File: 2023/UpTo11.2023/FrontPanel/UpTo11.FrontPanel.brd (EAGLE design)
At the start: 88 x 78 mm, 16 parts

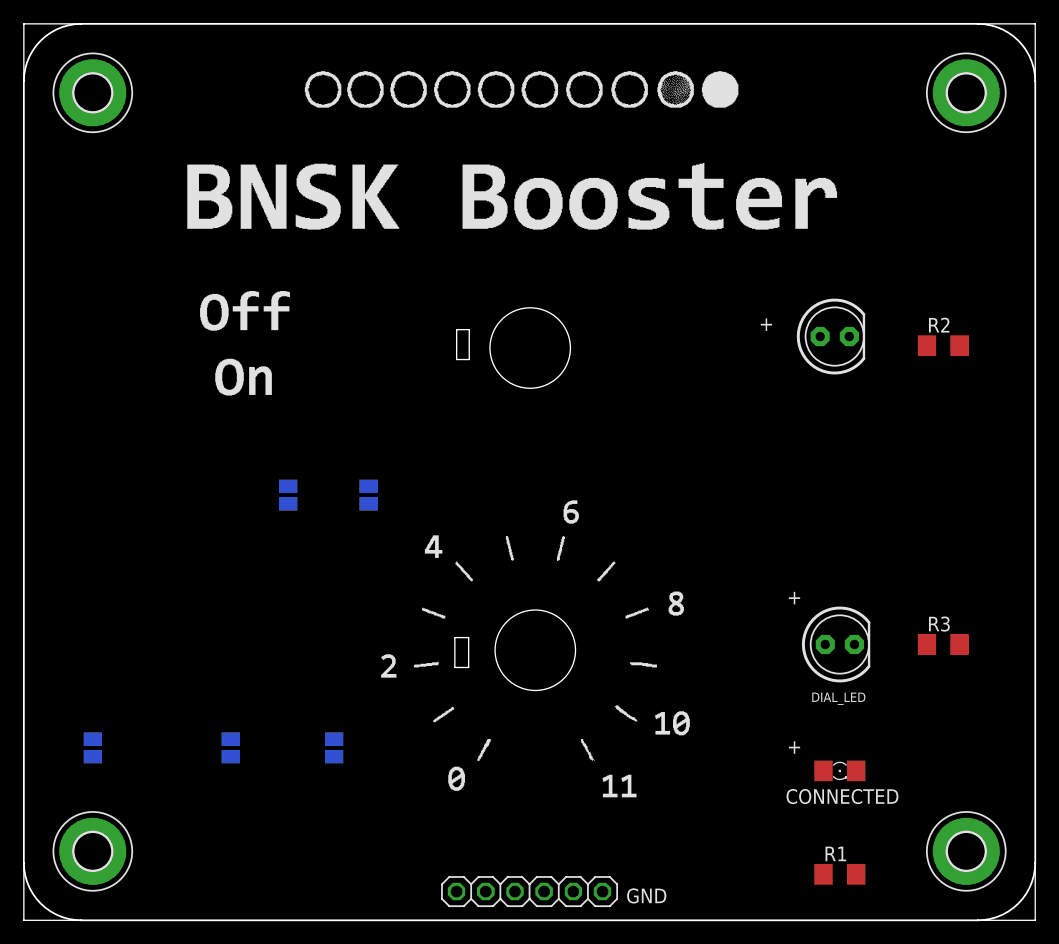
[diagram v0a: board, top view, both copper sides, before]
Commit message: BNSK Booster v 2
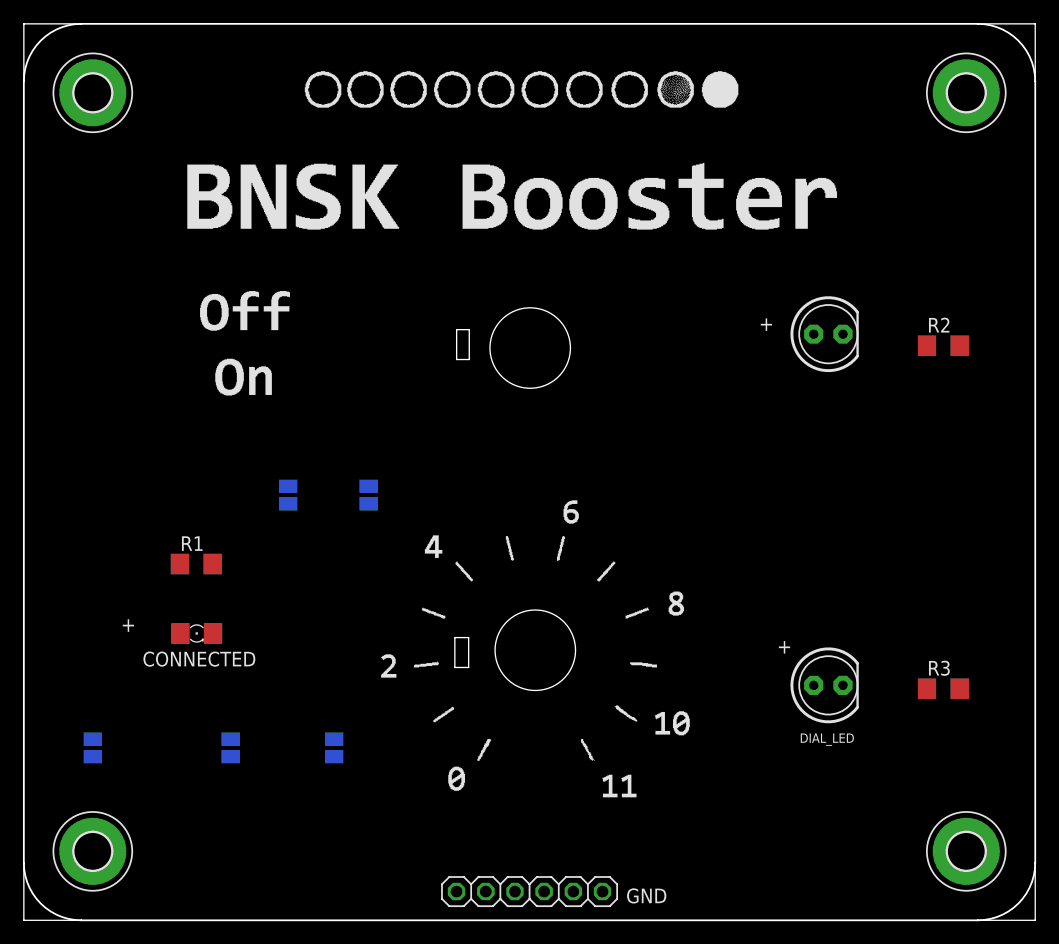
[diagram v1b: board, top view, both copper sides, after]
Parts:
- moved R1 62.2 mm to (17.0, 43.0)
- moved CONNECTED 57.2 mm to (17.0, 37.0)
- moved R3 3.85 mm to (82.0, 32.2)
- moved DIAL_LED 3.69 mm to (72.0, 32.4)
- moved BOOSTER_ON_LED 0.59 mm to (72.0, 63.0)
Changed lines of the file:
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@@
 <setting verticaltext="up"/>
 </settings>
-<grid distance="0.002857" unitdist="inch" unit="inch" style="dots" multiple="1" display="yes" altdistance="0.5" altunitdist="mm" altunit="mm"/>
+<grid distance="1" unitdist="mm" unit="mm" style="dots" multiple="1" display="yes" altdistance="0.5" altunitdist="mm" altunit="mm"/>
 <layers>
 <layer number="1" name="Top" color="4" fill="1" visible="yes" active="yes"/>
@@
 <rectangle x1="49.46501875" y1="48.41725" x2="50.16351875" y2="48.48075" layer="21"/>
 <rectangle x1="49.65551875" y1="48.48075" x2="50.16351875" y2="48.54425" layer="21"/>
-<text x="68.397859375" y="26.488084375" size="1.27" layer="21" font="vector">+</text>
+<text x="10.44090625" y="37.098934375" size="1.27" layer="21" font="vector">+</text>
 <text x="46.5" y="20" size="1.27" layer="26" rot="MR90" align="center">VCC_1K</text>
 <wire x1="2" y1="17" x2="2" y2="12" width="0" layer="20"/>
@@
 <wire x1="85" y1="12" x2="7" y2="12" width="0.1524" layer="20"/>
 <wire x1="7" y1="12" x2="2" y2="17" width="0.1524" layer="20" curve="-90"/>
-<text x="68.397859375" y="39.488084375" size="1.27" layer="21" font="vector">+</text>
+<text x="67.52704375" y="35.206584375" size="1.27" layer="21" font="vector">+</text>
 <rectangle x1="27.52851875" y1="82.70875" x2="28.54451875" y2="82.77225" layer="21"/>
 <rectangle x1="31.20898125" y1="82.70875" x2="32.22751875" y2="82.77225" layer="21"/>
@@
 <attribute name="VALUE" x="53.62" y="17.675" size="1.27" layer="27" rot="R180"/>
 </element>
-<element name="CONNECTED" library="adafruit" package="1206" value="" x="73" y="25" smashed="yes">
-<attribute name="NAME" x="73.23" y="22.77" size="1.27" layer="25" align="center"/>
-<attribute name="VALUE" x="71.73" y="22.46" size="1.27" layer="27"/>
+<element name="CONNECTED" library="adafruit" package="1206" value="" x="17.04305" y="36.9577375" smashed="yes">
+<attribute name="NAME" x="17.27305" y="34.7277375" size="1.27" layer="25" align="center"/>
+<attribute name="VALUE" x="15.77305" y="34.4177375" size="1.27" layer="27"/>
 </element>
-<element name="BOOSTER_ON_LED" library="adafruit" package="LED5MM" value="" x="72.5555" y="62.7935" smashed="yes">
-<attribute name="VALUE" x="75.7559" y="60.9901" size="1.27" layer="27" ratio="10"/>
+<element name="BOOSTER_ON_LED" library="adafruit" package="LED5MM" value="" x="72" y="63" smashed="yes">
+<attribute name="VALUE" x="75.2004" y="61.1966" size="1.27" layer="27" ratio="10"/>
 </element>
 <element name="POT_GND_(LEFT)" library="microbuilder" package="SOLDERJUMPER_REFLOW" value="" x="29" y="27" smashed="yes" rot="MR270">
@@
 <attribute name="VALUE" x="32" y="48.5999" size="0.02" layer="28" rot="MR270"/>
 </element>
-<element name="DIAL_LED" library="adafruit" package="LED5MM" value="" x="73" y="36" smashed="yes">
-<attribute name="NAME" x="70.5" y="31" size="0.8128" layer="25" ratio="10"/>
-<attribute name="VALUE" x="76.2004" y="34.1966" size="1.27" layer="27" ratio="10"/>
+<element name="DIAL_LED" library="adafruit" package="LED5MM" value="" x="72" y="32.444178125" smashed="yes">
+<attribute name="NAME" x="69.5" y="27.444178125" size="0.8128" layer="25" ratio="10"/>
+<attribute name="VALUE" x="75.2004" y="30.640778125" size="1.27" layer="27" ratio="10"/>
 </element>
 <element name="H1" library="holes" library_urn="urn:adsk.eagle:library:237" package="3,3-PAD" package3d_urn="urn:adsk.eagle:package:14283/1" value="MOUNT-PAD-ROUND3.3" x="8" y="84" smashed="yes">
@@
 <attribute name="POPULARITY" value="1" x="8" y="18" size="1.778" layer="27" display="off"/>
 </element>
-<element name="R1" library="adafruit" package="R1206" value="" x="73" y="16" smashed="yes">
-<attribute name="NAME" x="71.603" y="17.143" size="1.27" layer="25"/>
-<attribute name="VALUE" x="71.603" y="13.587" size="1.27" layer="27"/>
+<element name="R1" library="adafruit" package="R1206" value="" x="17" y="43" smashed="yes">
+<attribute name="NAME" x="15.603" y="44.143" size="1.27" layer="25"/>
+<attribute name="VALUE" x="15.603" y="40.587" size="1.27" layer="27"/>
 </element>
 <element name="R2" library="adafruit" package="R1206" value="" x="82" y="62" smashed="yes">
@@
 <attribute name="VALUE" x="80.603" y="59.587" size="1.27" layer="27"/>
 </element>
-<element name="R3" library="adafruit" package="R1206" value="" x="82" y="36" smashed="yes">
-<attribute name="NAME" x="80.603" y="37.143" size="1.27" layer="25"/>
-<attribute name="VALUE" x="80.603" y="33.587" size="1.27" layer="27"/>
+<element name="R3" library="adafruit" package="R1206" value="" x="82" y="32.15390625" smashed="yes">
+<attribute name="NAME" x="80.603" y="33.29690625" size="1.27" layer="25"/>
+<attribute name="VALUE" x="80.603" y="29.74090625" size="1.27" layer="27"/>
 </element>
 </elements>
@@
 <contactref element="R2" pad="1"/>
 <contactref element="R3" pad="1"/>
-<wire x1="80.578" y1="36" x2="80.578" y2="62" width="0" layer="19" extent="1-1"/>
-<wire x1="71.578" y1="16" x2="80.578" y2="36" width="0" layer="19" extent="1-1"/>
-<wire x1="52.35" y1="14.5" x2="71.578" y2="16" width="0" layer="19" extent="1-1"/>
+<wire x1="80.578" y1="32.15390625" x2="80.578" y2="62" width="0" layer="19" extent="1-1"/>
+<wire x1="52.35" y1="14.5" x2="80.578" y2="32.15390625" width="0" layer="19" extent="1-1"/>
 <wire x1="29" y1="26.238" x2="52.35" y2="14.5" width="0" layer="19" extent="16-16"/>
+<wire x1="15.578" y1="43" x2="29" y2="26.238" width="0" layer="19" extent="1-16"/>
 </signal>
 <signal name="DIAL_INPUT">
 <contactref element="POT_OUT_(MIDDLE)" pad="2"/>
 <contactref element="DIAL_LED" pad="A"/>
-<wire x1="20" y1="26.238" x2="71.73" y2="36" width="0" layer="19" extent="16-16"/>
+<wire x1="20" y1="26.238" x2="70.73" y2="32.444178125" width="0" layer="19" extent="16-16"/>
 </signal>
 <signal name="BOOSTER_ON">
@@
 <contactref element="POT_IN_(RIGHT)" pad="2"/>
 <contactref element="BOOSTER_ON_LED" pad="A"/>
-<wire x1="32" y1="48.238" x2="71.2855" y2="62.7935" width="0" layer="19" extent="16-16"/>
+<wire x1="32" y1="48.238" x2="70.73" y2="63" width="0" layer="19" extent="16-16"/>
 <wire x1="8" y1="26.238" x2="32" y2="48.238" width="0" layer="19" extent="16-16"/>
 </signal>
@@
 <contactref element="SWITCH_IN" pad="2"/>
 <contactref element="CONNECTED" pad="A"/>
-<wire x1="39.65" y1="14.5" x2="71.578" y2="25" width="0" layer="19" extent="1-1"/>
-<wire x1="25" y1="48.238" x2="39.65" y2="14.5" width="0" layer="19" extent="16-16"/>
+<wire x1="15.62105" y1="36.9577375" x2="25" y2="48.238" width="0" layer="19" extent="1-16"/>
+<wire x1="39.65" y1="14.5" x2="15.62105" y2="36.9577375" width="0" layer="19" extent="1-1"/>
 </signal>
 <signal name="N$1">
 <contactref element="R1" pad="2"/>
 <contactref element="CONNECTED" pad="C"/>
-<wire x1="74.422" y1="16" x2="74.422" y2="25" width="0" layer="19" extent="1-1"/>
+<wire x1="18.46505" y1="36.9577375" x2="18.422" y2="43" width="0" layer="19" extent="1-1"/>
 </signal>
 <signal name="N$2">
 <contactref element="R2" pad="2"/>
 <contactref element="BOOSTER_ON_LED" pad="K"/>
-<wire x1="73.8255" y1="62.7935" x2="83.422" y2="62" width="0" layer="19" extent="1-1"/>
+<wire x1="73.27" y1="63" x2="83.422" y2="62" width="0" layer="19" extent="1-1"/>
 </signal>
 <signal name="N$3">
 <contactref element="DIAL_LED" pad="K"/>
 <contactref element="R3" pad="2"/>
-<wire x1="74.27" y1="36" x2="83.422" y2="36" width="0" layer="19" extent="1-1"/>
+<wire x1="73.27" y1="32.444178125" x2="83.422" y2="32.15390625" width="0" layer="19" extent="1-1"/>
 </signal>
 </signals>

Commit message: UpTo11 2023 update
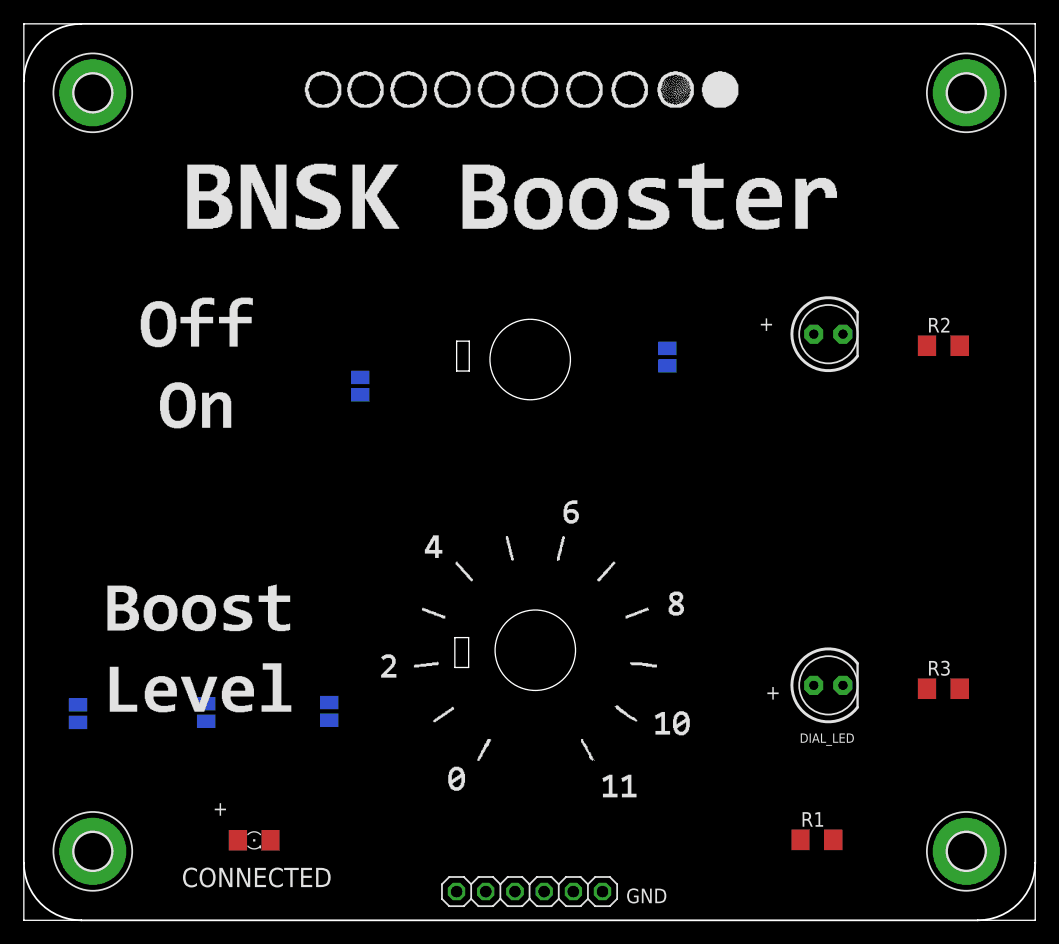
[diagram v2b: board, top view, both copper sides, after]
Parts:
- moved R1 59.1 mm to (71.0, 19.0)
- moved SWITCH_OUT 28.6 mm to (58.0, 61.0)
- moved CONNECTED 18.7 mm to (22.0, 19.0)
- moved SWITCH_IN 11.4 mm to (31.3, 58.5)
- moved POT_OUT_(MIDDLE) 3.75 mm to (17.9, 30.1)
- moved POT_IN_(RIGHT) 3.25 mm to (6.71, 30.0)
- moved POT_GND_(LEFT) 3.21 mm to (28.6, 30.2)
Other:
- outline, holes or cut-outs redrawn
